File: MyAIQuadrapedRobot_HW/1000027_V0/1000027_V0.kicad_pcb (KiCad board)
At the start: 2 copper layers, 40.1 x 43.8 mm, 4 parts, among them J1 10076801-406T18LF_9_by_2_head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, J2 0525591853, J3 MTSW-106-12-L-S-790_6_by_1_he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, J4 MOLEX_533750410

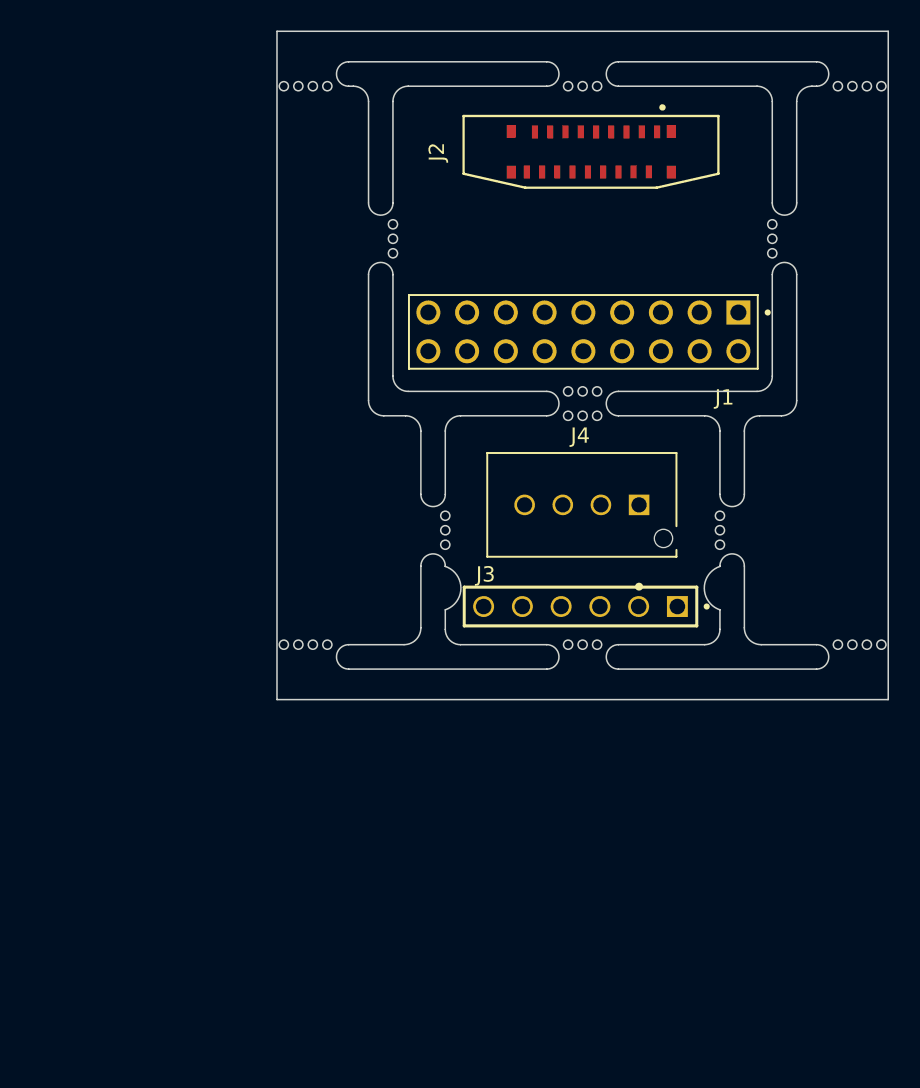
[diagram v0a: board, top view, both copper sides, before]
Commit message: 1000027_V0(a) ready for checking.
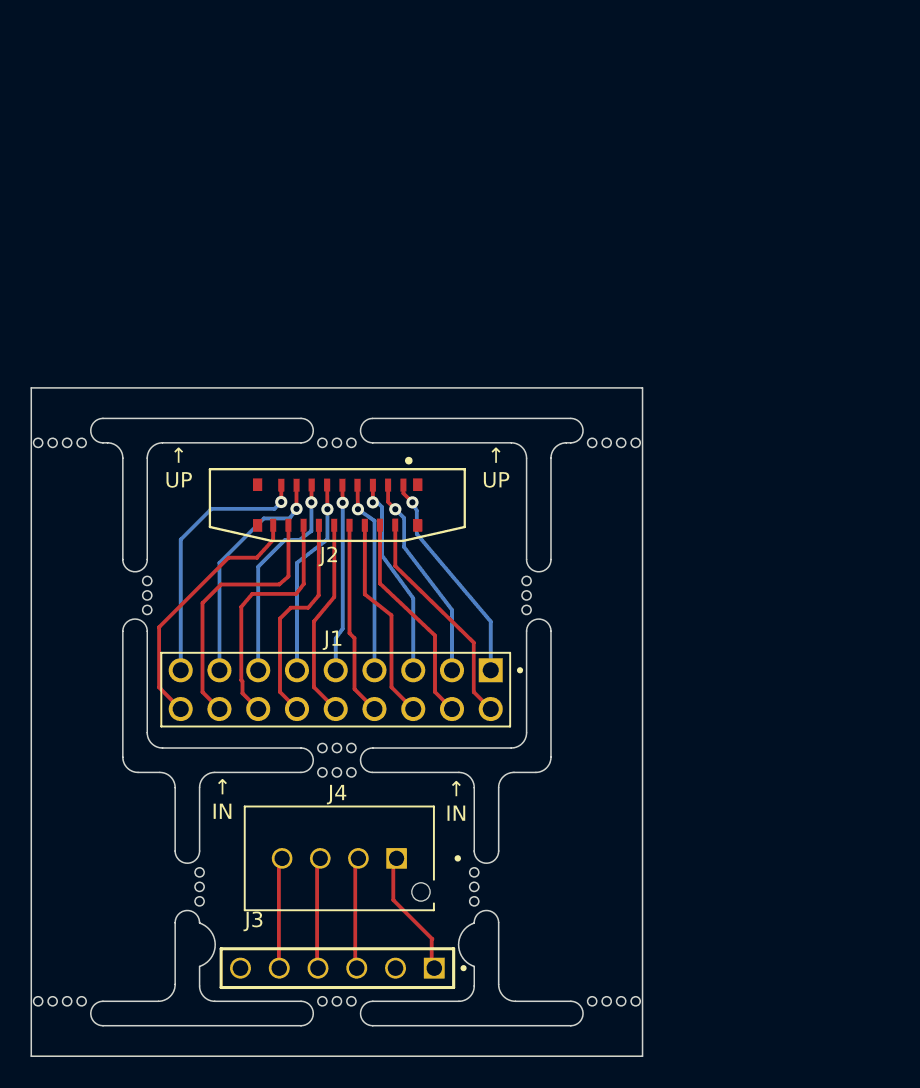
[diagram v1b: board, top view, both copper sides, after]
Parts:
- J4: value MOLEX_533750410 -> 533750410
- moved J3 28.6 mm to (149.5, 106.3)
- moved J1 28.5 mm to (149.4, 88.0)
- moved J2 28.5 mm to (149.3, 75.6)
- moved J4 28.1 mm to (153.4, 99.1)
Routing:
- net C17: track 0.00 -> 17.3 mm, vias 0 -> 1
- net C16: track 0.00 -> 17.1 mm
- net C18: track 0.00 -> 16.8 mm
- net C14: track 0.00 -> 15.8 mm
- net C15: track 0.00 -> 15.2 mm, vias 0 -> 1
- net C2: track 0.00 -> 14.7 mm
- net C1: track 0.00 -> 14.2 mm, vias 0 -> 1
- net C13: track 0.00 -> 14.2 mm, vias 0 -> 1
- net C12: track 0.00 -> 14.2 mm
- net C4: track 0.00 -> 14.0 mm
- net C3: track 0.00 -> 13.6 mm, vias 0 -> 1
- net C6: track 0.00 -> 13.5 mm
- net C5: track 0.00 -> 13.2 mm, vias 0 -> 1
- net C11: track 0.00 -> 13.1 mm, vias 0 -> 1
- net C10: track 0.00 -> 13.1 mm
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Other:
- outline, holes or cut-outs redrawn
- board text added: "1000027_V0a 1 of 2 Copyright © James Canova, June 2023, Victoria, BC Canada"
- board text added: "1000027_V0a 2 of 2 Copyright © James Canova, June 2023, Victoria, BC Canada"
- board text added: "↑ IN"
- board text added: "↑ UP"
